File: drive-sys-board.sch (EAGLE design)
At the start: 34 parts

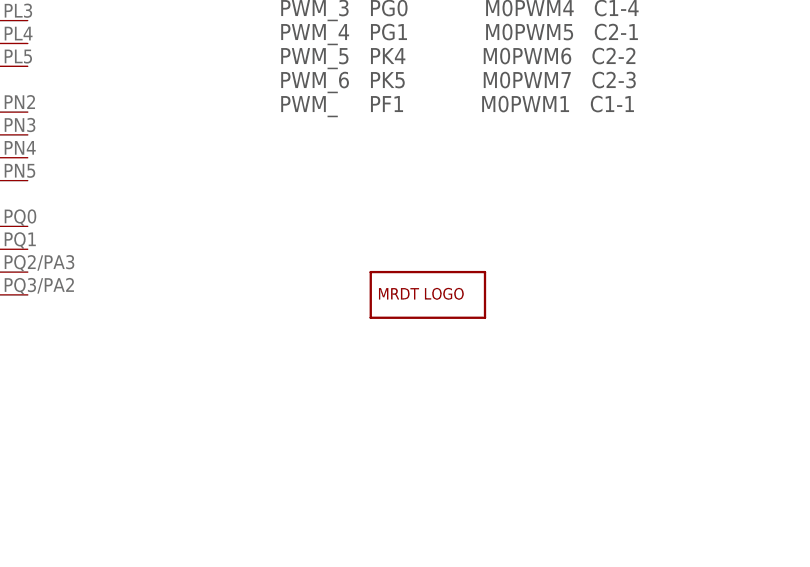
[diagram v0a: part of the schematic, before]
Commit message: finalized board
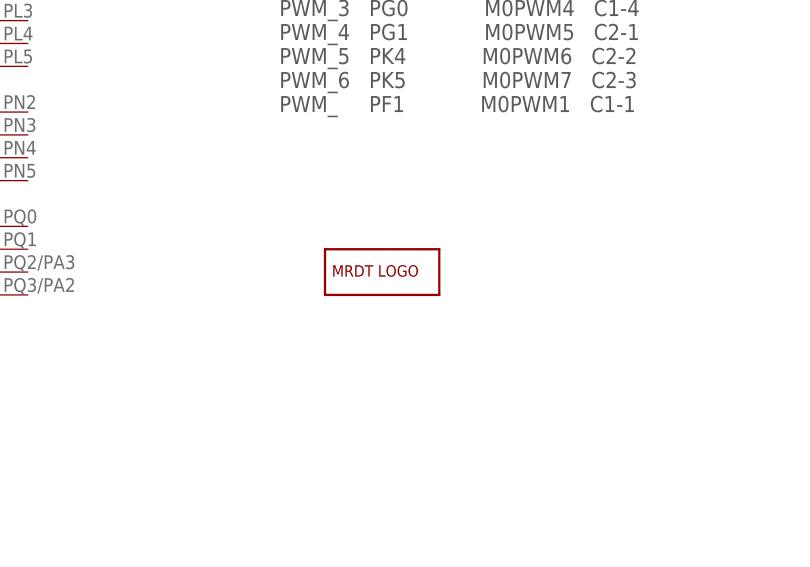
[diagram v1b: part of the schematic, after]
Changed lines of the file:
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@@
 <part name="H1" library="holes" deviceset="MOUNT-HOLE" device="3.2"/>
 <part name="U$7" library="MRDT-2015-General" deviceset="MLX-3-PIN" device=""/>
-<part name="U$8" library="MRDT-2015-General" deviceset="MRDT_LOGO" device=""/>
 <part name="U$10" library="MRDT-2015-General" deviceset="MAX3077" device=""/>
 <part name="U$11" library="MRDT-2015-General" deviceset="MAX3077" device=""/>
@@
 <part name="U$15" library="MRDT-2015-General" deviceset="MAX3077" device=""/>
 <part name="GND12" library="supply1" deviceset="GND" device=""/>
+<part name="U$8" library="MRDT-2015-General" deviceset="MRDT_LOGO" device=""/>
 </parts>
 <sheets>
@@
 <instance part="H1" gate="G$1" x="-5.08" y="-27.94"/>
 <instance part="U$7" gate="G$1" x="88.9" y="114.3"/>
-<instance part="U$8" gate="G$1" x="68.58" y="0"/>
 <instance part="U$10" gate="G$1" x="-101.6" y="106.68"/>
 <instance part="U$11" gate="G$1" x="-101.6" y="68.58"/>
@@
 <instance part="U$15" gate="G$1" x="-101.6" y="-83.82"/>
 <instance part="GND12" gate="1" x="-127" y="106.68"/>
+<instance part="U$8" gate="G$1" x="63.5" y="2.54"/>
 </instances>
 <busses>
@@
 </sheet>
 </sheets>
+<errors>
+</errors>
 </schematic>
 </drawing>
